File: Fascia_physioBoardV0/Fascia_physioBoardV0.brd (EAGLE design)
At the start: 37.9 x 40 mm, 88 parts, among them CN2 CA0612KRX7R9BB102, CN3 CA0612KRX7R9BB102, CN4 CA0612KRX7R9BB102, CN5 CA0612KRX7R9BB102, CN6 CA0612KRX7R9BB102, J1 MOLEX_52437-2471MOLEX_52437-2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, J2 MOLEX_52437-2471MOLEX_52437-2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, J3 MOLEX_51296-1294MOLEX_51296-1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, U1 ADS1299-X, U10 TPD4E1B06DCKR, U11 TPD4E1B06DCKR, U12 OPA320AIDBVRDBV5-L, U13 ADUM5028, U2 OPA2320AIDGKT_NOVA8-SOIC-L, U3 OPA2320AIDGKT_NOVAL8-SOIC-L, U4 HCNR200-300E, U5 OPA320AIDBVRDBV5-L, U6 TPD4E1B06DCKR, U7 TPD4E1B06DCKR, U8 TPD4E1B06DCKR, U9 TPD4E1B06DCKR

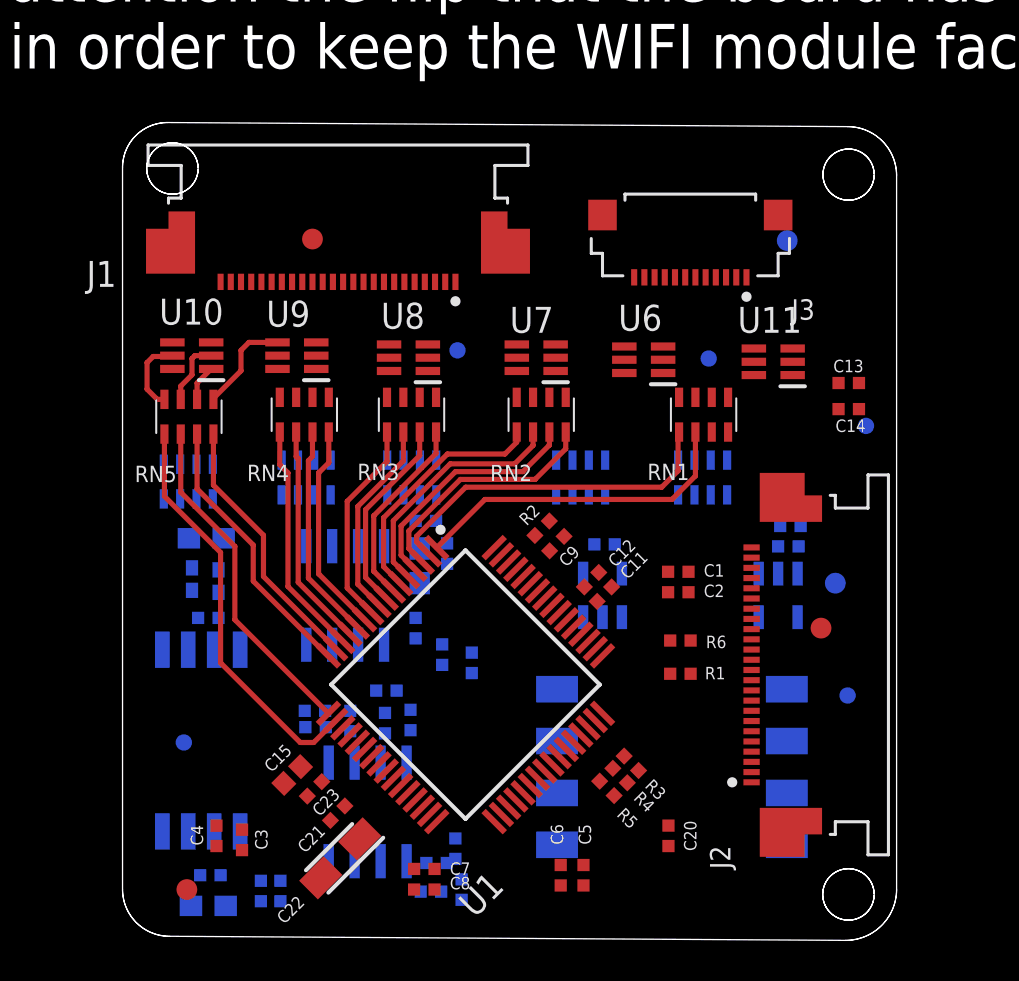
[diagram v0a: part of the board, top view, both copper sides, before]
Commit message: minor layout changes
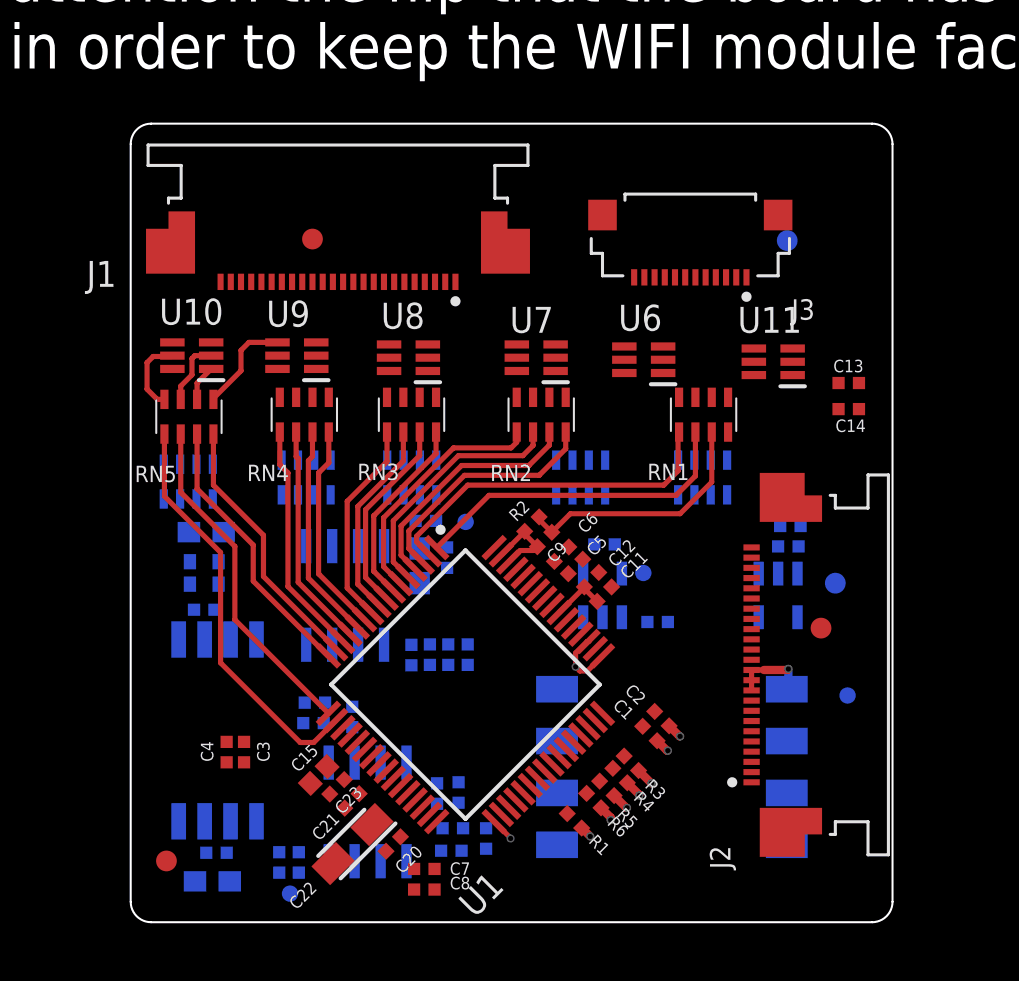
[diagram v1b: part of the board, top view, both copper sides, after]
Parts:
- moved C6 15.7 mm to (23.8, 19.2), turned to 225 degrees
- moved C5 15.1 mm to (24.5, 18.6), turned to 45 degrees
- moved R16 14.9 mm to (28.5, 15.9), turned to 180 degrees
- moved C20 13.5 mm to (15.6, 5.03), turned to 225 degrees
- moved DVDD_ISO 11.0 mm to (27.8, 18.3)
- moved RAW_EDA_SIG 9.04 mm to (10.5, 2.60)
- moved R6 8.91 mm to (25.4, 7.15), turned to 135 degrees
- moved R1 8.87 mm to (24.4, 6.16), turned to 135 degrees
- moved GND_ISO 8.41 mm to (19.1, 20.8)
- moved C1 8.04 mm to (28.1, 10.4), turned to 135 degrees
- moved C2 6.24 mm to (28.7, 11.2), turned to 135 degrees
- moved PA02_EDA_SIG 5.66 mm to (34.5, 21.7)
- moved C30 4.95 mm to (18.8, 7.55)
- moved C3 4.30 mm to (8.25, 9.53)
- moved C4 4.13 mm to (7.40, 9.53)
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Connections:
- net AVDD: now also U11.2
- net VCC: no longer U11.2
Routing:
- net GND: track 0.00 -> 13.2 mm, vias 0 -> 9
- net BIAS_DRV: track 0.00 -> 12.3 mm
- net N$17: track 0.00 -> 4.30 mm
- net N$63: track 0.00 -> 2.73 mm
- net AGND: track 0.00 -> 0.59 mm, vias 0 -> 1
- added copper zone on layer 2, net AGND
- added copper zone on layer 2, net GND
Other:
- board size 37.9 x 40 mm -> 37.3 x 39.1 mm
